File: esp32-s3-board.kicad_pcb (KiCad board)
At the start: 2 copper layers, 65 x 45 mm, 57 parts, among them J1 USB_C_Receptacle_USB2.0_14P, J2 OV2640, J3 Micro_SD_Card, J4 Conn_01x08, SW1 BOOT_SW, SW2 RST_SW, U1 ESP32-S3, U2 MCP1700x-280xxTT, U3 W25Q128JVS, U4 ESP-PSRAM64H, U6 NCP1117-1.5_SOT223, U7 MCP1700x-330xxTT, Y1 40MHz

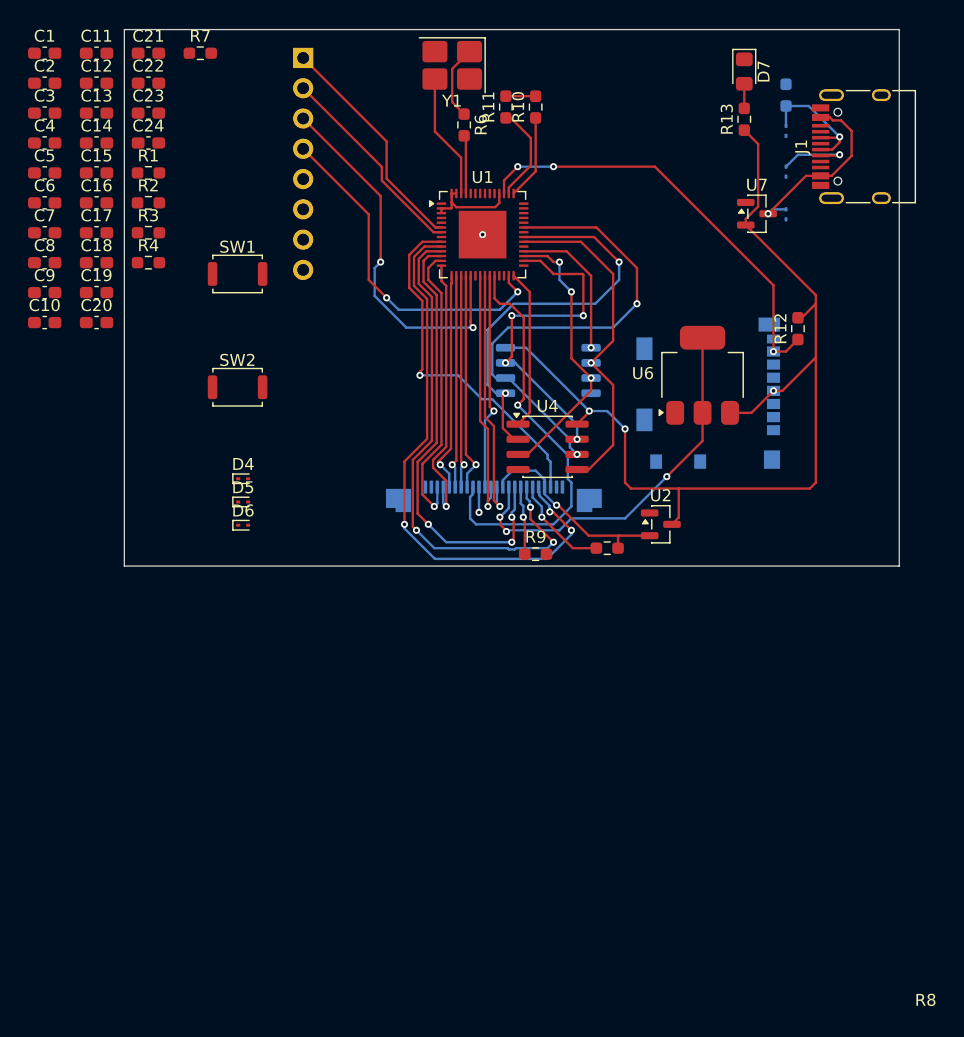
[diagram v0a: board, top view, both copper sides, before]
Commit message: Finished routing pcb
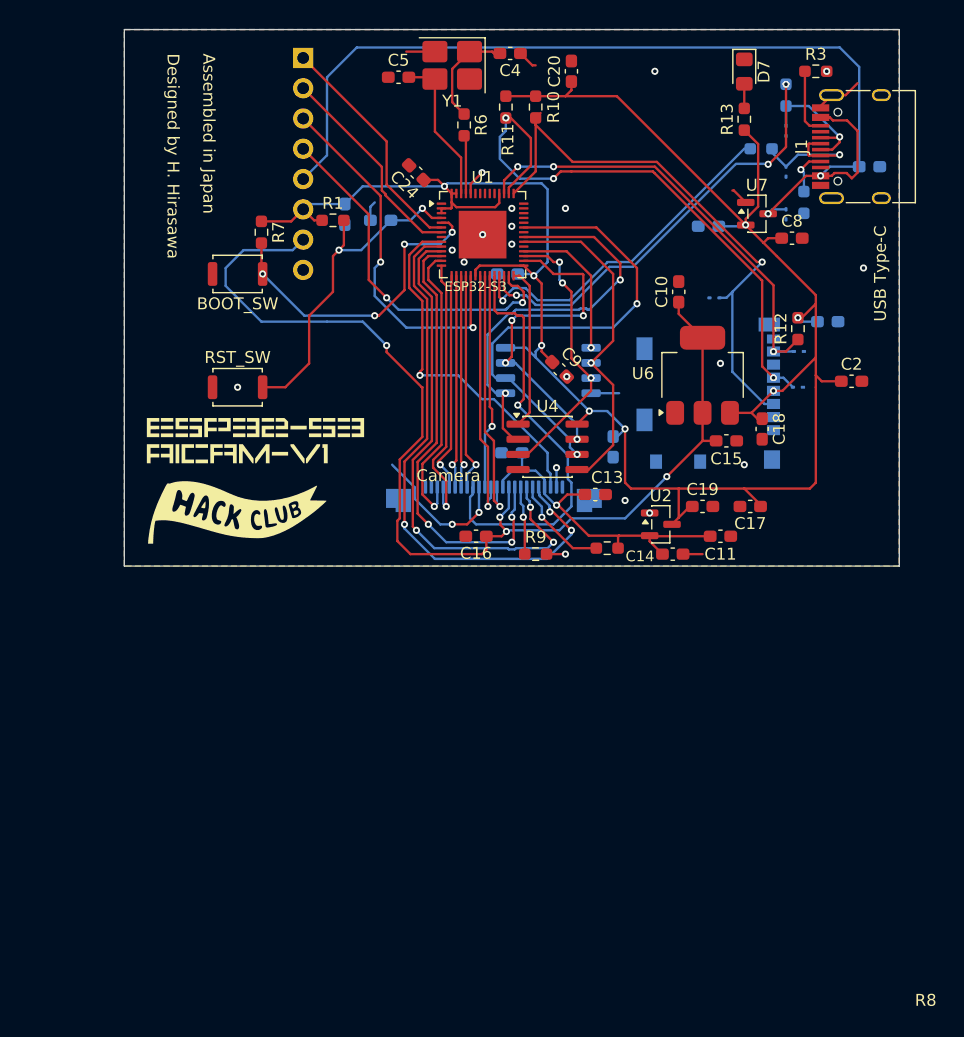
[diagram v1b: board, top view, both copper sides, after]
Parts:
- added G***: LOGO, logos:hackclub, F.Cu at (120.5, 91.5)
- added G***: LOGO, logos:hackclub, F.Cu at (124.5, 95.5)
- added G***: LOGO, LOGO, F.Cu at (127.6, 93.2)
- C1, C12, C21, C22, C23, C3, C6, C7, D4, D5, D6, R2, R4: moved to B.Cu
- moved C2 72.2 mm to (176.0, 84.5)
- moved C1 69.8 mm to (177.5, 66.5)
- moved C11 66.2 mm to (165.0, 97.5)
- moved C8 62.7 mm to (171.0, 72.5)
- moved C23 59.6 mm to (174.0, 79.5)
- moved C17 59.4 mm to (167.5, 95.0), turned to 180 degrees
- moved C14 59.4 mm to (161.0, 99.0)
- moved R3 57.6 mm to (173.0, 58.5)
- moved C18 57.5 mm to (168.5, 88.5), turned to -90 degrees
- moved C15 57.4 mm to (165.5, 89.5)
- moved C6 55.7 mm to (164.0, 71.5), turned to 180 degrees
- moved R2 55.0 mm to (172.0, 69.5), turned to -90 degrees
- moved C19 53.9 mm to (163.5, 95.0)
- moved C10 53.2 mm to (161.5, 77.0), turned to 90 degrees
- moved C13 52.7 mm to (154.5, 94.0)
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- renumbered SW1 to BOOT_SW, SW2 to RST_SW
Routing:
- net +3V3: track 93.0 -> 185.0 mm, vias 3 -> 8
- net +5V: track 15.8 -> 85.6 mm, vias 1 -> 2
- net DVDD_1V5: track 32.6 -> 91.7 mm, vias 3 -> 4
- net IO38: track 7.10 -> 48.1 mm, vias 0 -> 1
- net IO39: track 8.21 -> 49.1 mm, vias 0 -> 3
- net Net-(U1-GPIO20/USB_D+): track 0.00 -> 36.1 mm, vias 0 -> 3
- net GND: track 2.12 -> 33.1 mm, vias 2 -> 21
- net Net-(U1-GPIO19/USB_D-): track 0.00 -> 29.2 mm, vias 0 -> 1
- net Net-(U1-CHIP_PU): track 0.00 -> 28.3 mm, vias 0 -> 2
- net Net-(U1-GPIO0): track 0.00 -> 26.7 mm, vias 0 -> 4
- net AVDD_2V8: track 17.3 -> 28.7 mm
- net Net-(J1-CC2): track 0.00 -> 5.66 mm
- net D-: track 6.54 -> 11.5 mm
- net Net-(J1-CC1): track 0.00 -> 3.88 mm, vias 0 -> 1
- net Net-(C4-Pad2): track 6.25 -> 8.86 mm
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- added copper zone on B.Cu, net GND
- added copper zone on F.Cu, net GND
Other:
- board text added: "Assembled in Japan"
- board text added: "Camera"
- board text added: "Designed by H. Hirasawa"
- board text added: "ESP32-S3"
- board text added: "USB Type-C"
